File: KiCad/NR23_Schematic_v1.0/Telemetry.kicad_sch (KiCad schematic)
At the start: 1 part

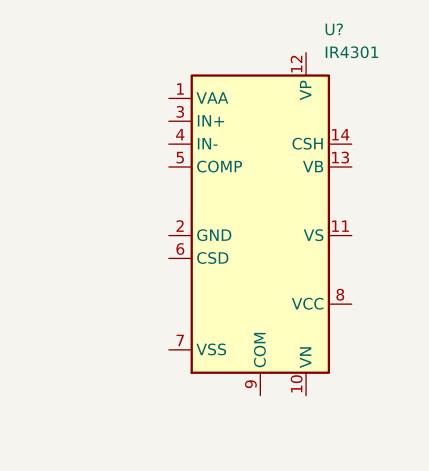
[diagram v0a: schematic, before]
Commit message: zig
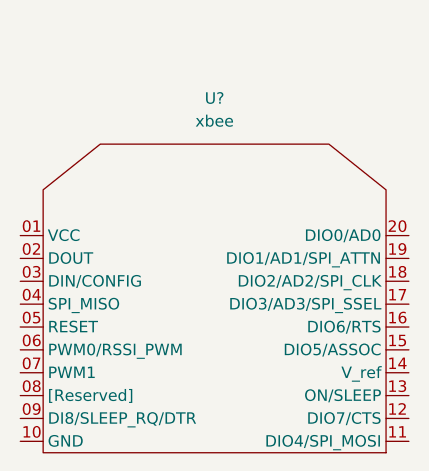
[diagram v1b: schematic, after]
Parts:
- removed U?: IR4301, Package_DFN_QFN:Infineon_PQFN-22-15-4EP_6x5mm_P0.65mm, symbol Amplifier_Audio:IR4301
- added U?: xbee, symbol Homssymbols:xbee
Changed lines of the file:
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@@
 (kicad_sch (version 20211123) (generator eeschema)
   (paper "A4")
-  (symbol (lib_id "Amplifier_Audio:IR4301") (at 121.92 78.74 0) (unit 1)
+  (symbol (lib_id "Homssymbols:xbee") (at 83.82 106.68 0) (unit 1)
     (in_bom yes) (on_board yes) (fields_autoplaced)
-    (property "Reference" "U?" (id 0) (at 129.0194 55.88 0)
-      (effects (font (size 1.27 1.27)) (justify left))
-    )
-    (property "Value" "IR4301" (id 1) (at 129.0194 58.42 0)
-      (effects (font (size 1.27 1.27)) (justify left))
-    )
-    (property "Footprint" "Package_DFN_QFN:Infineon_PQFN-22-15-4EP_6x5mm_P0.65mm" (id 2) (at 121.92 78.74 0)
-      (effects (font (size 1.27 1.27) italic) hide)
-    )
-    (property "Datasheet" "https://www.infineon.com/dgdl/ir4301.pdf?fileId=5546d462533600a4015355d5fc691819" (id 3) (at 121.92 78.74 0)
+    (property "Reference" "U?" (id 0) (at 116.84 63.5 0))
+    (property "Value" "xbee" (id 1) (at 116.84 66.04 0))
+    (property "Footprint" "" (id 2) (at 83.82 106.68 0)
       (effects (font (size 1.27 1.27)) hide)
     )
-    (pin "1")
+    (property "Datasheet" "" (id 3) (at 83.82 106.68 0)
+      (effects (font (size 1.27 1.27)) hide)
+    )
+    (pin "01")
+    (pin "02")
+    (pin "03")
+    (pin "04")
+    (pin "05")
+    (pin "06")
+    (pin "07")
+    (pin "08")
+    (pin "09")
     (pin "10")
     (pin "11")
@@
     (pin "14")
     (pin "15")
-    (pin "2")
-    (pin "3")
-    (pin "4")
-    (pin "5")
-    (pin "6")
-    (pin "7")
-    (pin "8")
-    (pin "9")
+    (pin "16")
+    (pin "17")
+    (pin "18")
+    (pin "19")
+    (pin "20")
   )
 )
